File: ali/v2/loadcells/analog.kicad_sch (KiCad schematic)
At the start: 40 parts, among them J10 Conn_01x04, J11 Conn_01x04, J12 Conn_01x04, J9 Conn_01x04, U6 ADS124S08

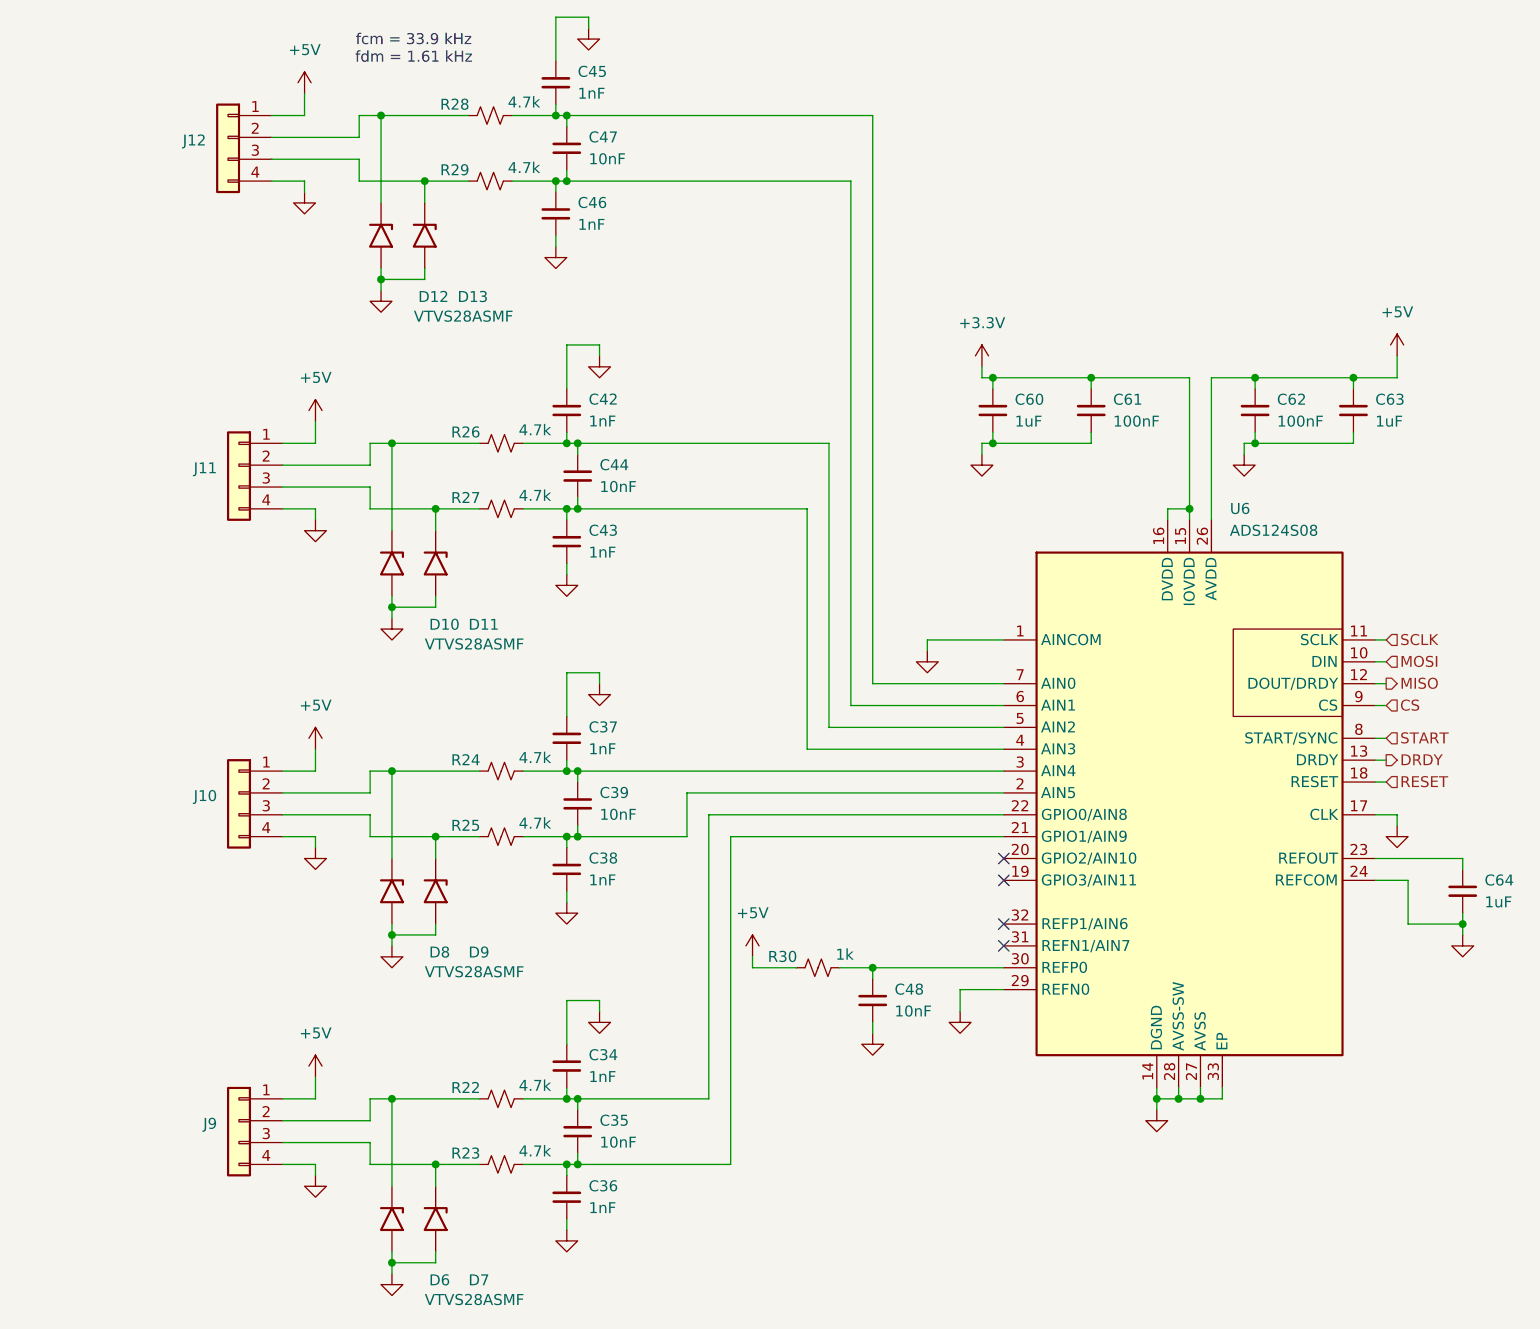
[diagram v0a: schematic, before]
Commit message: Small cleanups
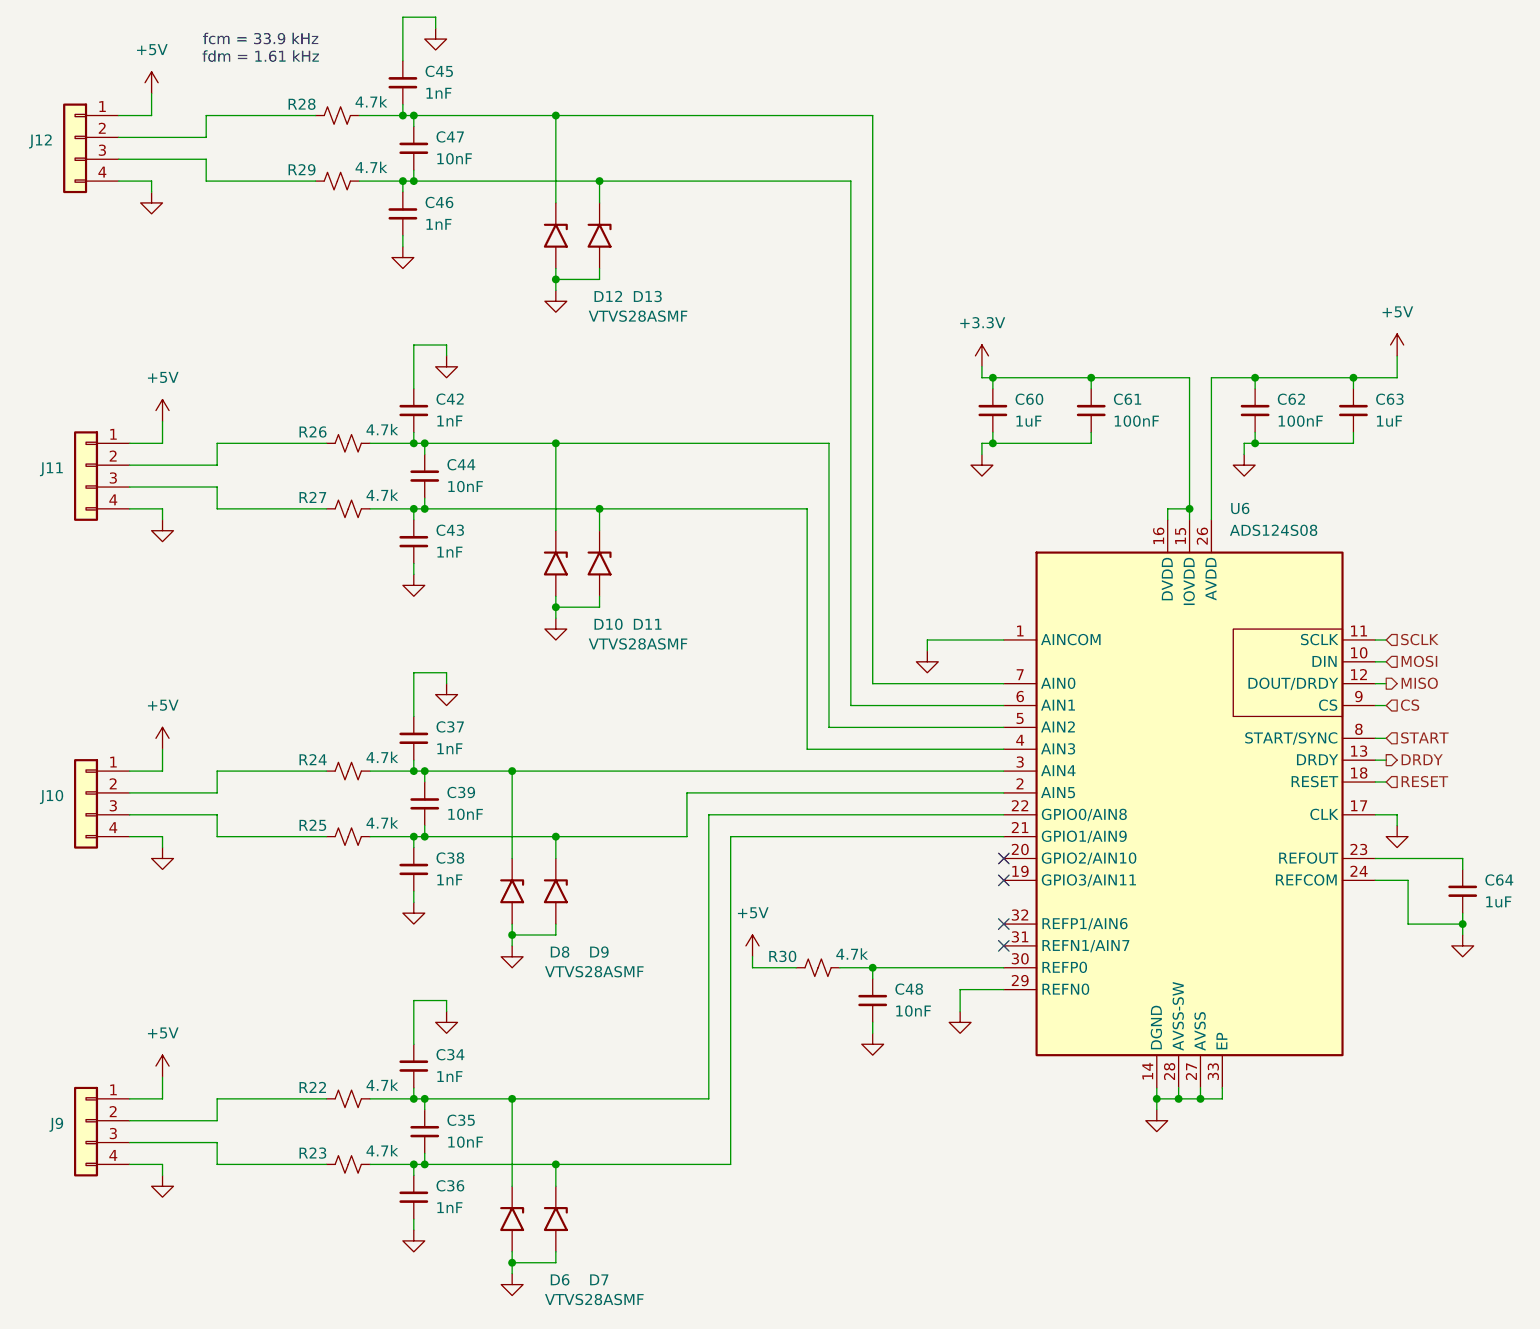
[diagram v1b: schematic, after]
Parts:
- R30: value 1k -> 4.7k; MPN RT0603BRD071KL -> RT0603BRD074K7L
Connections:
- net at C38.2, C39.1, R25.2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: now also D9.1 (A1)
- net at C34.1, C35.2, R22.2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: now also D6.1 (A1)
- net at J9.3 (Pin_3), R23.1: no longer D7.1 (A1)
- net at C35.1, C36.2, R23.2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: now also D7.1 (A1)
- net at J11.2 (Pin_2), R26.1: no longer D10.1 (A1)
- net at J11.3 (Pin_3), R27.1: no longer D11.1 (A1)
- net at J12.2 (Pin_2), R28.1: no longer D12.1 (A1)
- net at C45.1, C47.2, R28.2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: now also D12.1 (A1)
- net at C37.1, C39.2, R24.2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: now also D8.1 (A1)
- net at J10.3 (Pin_3), R25.1: no longer D9.1 (A1)
- net at J12.3 (Pin_3), R29.1: no longer D13.1 (A1)
- net at C43.2, C44.1, R27.2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: now also D11.1 (A1)
- net at J9.2 (Pin_2), R22.1: no longer D6.1 (A1)
- net at J10.2 (Pin_2), R24.1: no longer D8.1 (A1)
- net at C46.2, C47.1, R29.2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: now also D13.1 (A1)
- net at C42.1, C44.2, R26.2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: now also D10.1 (A1)
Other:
- moved on the sheet: C34, C35, C36, C37, C38, C39, C42, C43, C44, C45, C46, C47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
